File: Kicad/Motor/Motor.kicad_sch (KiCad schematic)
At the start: 7 parts, among them J1 12V, J2 PWM, J3 Motor 12V, J4 Motor Ground, J5 Ground, Q1 TIP120

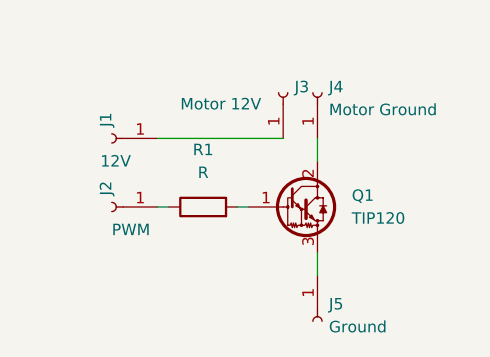
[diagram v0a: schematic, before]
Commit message: Update
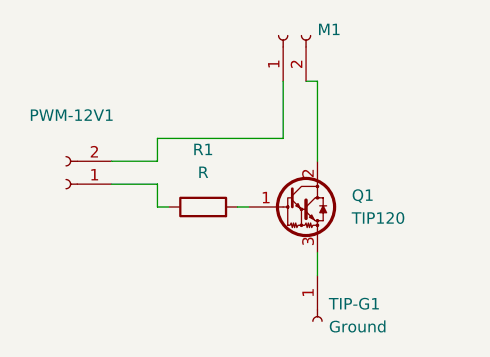
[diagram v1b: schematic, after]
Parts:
- removed J1: 12V, Connector_PinHeader_1.00mm:PinHeader_1x01_P1.00mm_Vertical, symbol Connector:Conn_01x01_Female
- removed J2: PWM, Connector_PinHeader_1.00mm:PinHeader_1x01_P1.00mm_Vertical, symbol Connector:Conn_01x01_Female
- removed J3: Motor 12V, Connector_PinHeader_1.00mm:PinHeader_1x01_P1.00mm_Vertical, symbol Connector:Conn_01x01_Female
- removed J4: Motor Ground, Connector_PinHeader_1.00mm:PinHeader_1x01_P1.00mm_Vertical, symbol Connector:Conn_01x01_Female
- added M1, PWM-12V1: (no value), symbol Connector:Conn_01x02_Female
- TIP-G1: renamed from J5; footprint (none) -> Connector_PinHeader_1.00mm:PinHeader_1x01_P1.00mm_Vertical
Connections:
- net at R1.1: now also PWM-12V1.1 (Pin_1)
- net at Q1.2 (C): now also M1.2 (Pin_2)
- new net: M1.1 (Pin_1), PWM-12V1.2 (Pin_2)
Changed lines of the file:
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@@
+    (stroke (width 0) (type default) (color 0 0 0 0))
+  )
+  (wire (pts (xy 135.89 86.36) (xy 134.62 86.36))
+    (stroke (width 0) (type default) (color 0 0 0 0))
+  )
+  (wire (pts (xy 118.11 95.25) (xy 118.11 92.71))
     (stroke (width 0) (type default) (color 0 0 0 0))
   )
   (wire (pts (xy 118.11 100.33) (xy 119.38 100.33))
+    (stroke (width 0) (type default) (color 0 0 0 0))
+  )
+  (wire (pts (xy 113.03 97.79) (xy 118.11 97.79))
+    (stroke (width 0) (type default) (color 0 0 0 0))
+  )
+  (wire (pts (xy 118.11 97.79) (xy 118.11 100.33))
     (stroke (width 0) (type default) (color 0 0 0 0))
   )
@@
     (stroke (width 0) (type default) (color 0 0 0 0))
   )
-  (wire (pts (xy 135.89 92.71) (xy 135.89 95.25))
+  (wire (pts (xy 113.03 95.25) (xy 118.11 95.25))
     (stroke (width 0) (type default) (color 0 0 0 0))
   )
-  (symbol (lib_id "Connector:Conn_01x01_Female") (at 113.03 100.33 180) (unit 1)
-    (in_bom yes) (on_board yes)
-    (property "Reference" "J2" (id 0) (at 112.3949 99.06 90)
-      (effects (font (size 1.27 1.27)) (justify right))
-    )
-    (property "Value" "PWM" (id 1) (at 113.03 102.87 0)
-      (effects (font (size 1.27 1.27)) (justify right))
-    )
-    (property "Footprint" "Connector_PinHeader_1.00mm:PinHeader_1x01_P1.00mm_Vertical" (id 2) (at 113.03 100.33 0)
-      (effects (font (size 1.27 1.27)) hide)
-    )
-    (property "Datasheet" "~" (id 3) (at 113.03 100.33 0)
-      (effects (font (size 1.27 1.27)) hide)
-    )
-    (pin "1")
+  (wire (pts (xy 135.89 86.36) (xy 135.89 95.25))
+    (stroke (width 0) (type default) (color 0 0 0 0))
+  )
+  (wire (pts (xy 132.08 86.36) (xy 132.08 92.71))
+    (stroke (width 0) (type default) (color 0 0 0 0))
   )
   (symbol (lib_id "Device:R") (at 123.19 100.33 90) (unit 1)
@@
     (pin "2")
   )
-  (symbol (lib_id "Connector:Conn_01x01_Female") (at 132.08 87.63 90) (unit 1)
+  (symbol (lib_id "Connector:Conn_01x02_Female") (at 107.95 97.79 180) (unit 1)
     (in_bom yes) (on_board yes)
-    (property "Reference" "J3" (id 0) (at 133.35 86.9949 90)
-      (effects (font (size 1.27 1.27)) (justify right))
-    )
-    (property "Value" "Motor 12V" (id 1) (at 120.65 88.9 90)
-      (effects (font (size 1.27 1.27)) (justify right))
-    )
-    (property "Footprint" "Connector_PinHeader_1.00mm:PinHeader_1x01_P1.00mm_Vertical" (id 2) (at 132.08 87.63 0)
+    (property "Reference" "PWM-12V1" (id 0) (at 108.585 90.17 0))
+    (property "Value" "" (id 1) (at 107.95 92.71 0))
+    (property "Footprint" "" (id 2) (at 107.95 97.79 0)
       (effects (font (size 1.27 1.27)) hide)
     )
-    (property "Datasheet" "~" (id 3) (at 132.08 87.63 0)
+    (property "Datasheet" "~" (id 3) (at 107.95 97.79 0)
       (effects (font (size 1.27 1.27)) hide)
     )
     (pin "1")
-  )
-  (symbol (lib_id "Connector:Conn_01x01_Female") (at 135.89 87.63 90) (unit 1)
-    (in_bom yes) (on_board yes) (fields_autoplaced)
-    (property "Reference" "J4" (id 0) (at 137.16 86.9949 90)
-      (effects (font (size 1.27 1.27)) (justify right))
-    )
-    (property "Value" "Motor Ground" (id 1) (at 137.16 89.5349 90)
-      (effects (font (size 1.27 1.27)) (justify right))
-    )
-    (property "Footprint" "Connector_PinHeader_1.00mm:PinHeader_1x01_P1.00mm_Vertical" (id 2) (at 135.89 87.63 0)
-      (effects (font (size 1.27 1.27)) hide)
-    )
-    (property "Datasheet" "~" (id 3) (at 135.89 87.63 0)
-      (effects (font (size 1.27 1.27)) hide)
-    )
-    (pin "1")
-  )
-  (symbol (lib_id "Connector:Conn_01x01_Female") (at 113.03 92.71 180) (unit 1)
-    (in_bom yes) (on_board yes)
-    (property "Reference" "J1" (id 0) (at 112.3949 91.44 90)
-      (effects (font (size 1.27 1.27)) (justify right))
-    )
-    (property "Value" "12V" (id 1) (at 111.76 95.25 0)
-      (effects (font (size 1.27 1.27)) (justify right))
-    )
-    (property "Footprint" "Connector_PinHeader_1.00mm:PinHeader_1x01_P1.00mm_Vertical" (id 2) (at 113.03 92.71 0)
-      (effects (font (size 1.27 1.27)) hide)
-    )
-    (property "Datasheet" "~" (id 3) (at 113.03 92.71 0)
-      (effects (font (size 1.27 1.27)) hide)
-    )
-    (pin "1")
+    (pin "2")
   )
   (symbol (lib_id "Transistor_BJT:TIP120") (at 133.35 100.33 0) (unit 1)
@@
   (symbol (lib_id "Connector:Conn_01x01_Female") (at 135.89 113.03 270) (unit 1)
     (in_bom yes) (on_board yes) (fields_autoplaced)
-    (property "Reference" "J5" (id 0) (at 137.16 111.1249 90)
+    (property "Reference" "TIP-G1" (id 0) (at 137.16 111.1249 90)
       (effects (font (size 1.27 1.27)) (justify left))
     )
@@
       (effects (font (size 1.27 1.27)) (justify left))
     )
-    (property "Footprint" "" (id 2) (at 135.89 113.03 0)
+    (property "Footprint" "Connector_PinHeader_1.00mm:PinHeader_1x01_P1.00mm_Vertical" (id 2) (at 135.89 113.03 0)
       (effects (font (size 1.27 1.27)) hide)
     )
@@
     (pin "1")
   )
+  (symbol (lib_id "Connector:Conn_01x02_Female") (at 132.08 81.28 90) (unit 1)
+    (in_bom yes) (on_board yes) (fields_autoplaced)
+    (property "Reference" "M1" (id 0) (at 135.89 80.6449 90)
+      (effects (font (size 1.27 1.27)) (justify right))
+    )
+    (property "Value" "" (id 1) (at 135.89 83.1849 90)
+      (effects (font (size 1.27 1.27)) (justify right))
+    )
+    (property "Footprint" "" (id 2) (at 132.08 81.28 0)
+      (effects (font (size 1.27 1.27)) hide)
+    )
+    (property "Datasheet" "~" (id 3) (at 132.08 81.28 0)
+      (effects (font (size 1.27 1.27)) hide)
+    )
+    (pin "1")
+    (pin "2")
+  )
   (sheet_instances
     (path "/" (page "1"))
   )
   (symbol_instances
-    (path "/7c62ca8e-341b-47b7-a6ac-146619cf8af7"
-      (reference "J1") (unit 1) (value "12V") (footprint "Connector_PinHeader_1.00mm:PinHeader_1x01_P1.00mm_Vertical")
+    (path "/d94772bc-24d5-4084-a116-79cfd5ce463b"
+      (reference "M1") (unit 1) (value "M 12V og M Gorund") (footprint "Connector_PinHeader_1.00mm:PinHeader_1x02_P1.00mm_Vertical")
     )
-    (path "/44b5b889-9513-4d19-bee0-2686c873ad91"
-      (reference "J2") (unit 1) (value "PWM") (footprint "Connector_PinHeader_1.00mm:PinHeader_1x01_P1.00mm_Vertical")
-    )
-    (path "/667630b3-d30f-46f8-8e3e-857bb26f7e4c"
-      (reference "J3") (unit 1) (value "Motor 12V") (footprint "Connector_PinHeader_1.00mm:PinHeader_1x01_P1.00mm_Vertical")
-    )
-    (path "/694f9512-3fbb-423c-aeb8-3d6bc1068fd8"
-      (reference "J4") (unit 1) (value "Motor Ground") (footprint "Connector_PinHeader_1.00mm:PinHeader_1x01_P1.00mm_Vertical")
-    )
-    (path "/c808e14d-35bb-4517-9734-9a810eb055dd"
-      (reference "J5") (unit 1) (value "Ground") (footprint "Connector_PinHeader_1.00mm:PinHeader_1x01_P1.00mm_Vertical")
+    (path "/4f46b8e8-9e73-4b6a-8e59-fbe50391f07b"
+      (reference "PWM-12V1") (unit 1) (value "PWM og 12V") (footprint "Connector_PinHeader_1.00mm:PinHeader_1x02_P1.00mm_Vertical")
     )
     (path "/98d35d65-4330-40a9-ba56-7f42d94d101d"
@@
       (reference "R1") (unit 1) (value "R") (footprint "Resistor_THT:R_Axial_DIN0204_L3.6mm_D1.6mm_P7.62mm_Horizontal")
     )
+    (path "/c808e14d-35bb-4517-9734-9a810eb055dd"
+      (reference "TIP-G1") (unit 1) (value "Ground") (footprint "Connector_PinHeader_1.00mm:PinHeader_1x01_P1.00mm_Vertical")
+    )
   )
